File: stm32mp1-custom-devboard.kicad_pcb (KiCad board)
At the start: 4 copper layers, 120 x 72 mm, 50 parts, among them Con1 52746-0671, Con2 505110-2491, Con3 2041119-1, U1 TPS61169DCKR, U2 MCP1703T-3302E, U3 ST1S10PHR, U4 ST1S09IPUR, U5 STM32F103C(8-B)Tx

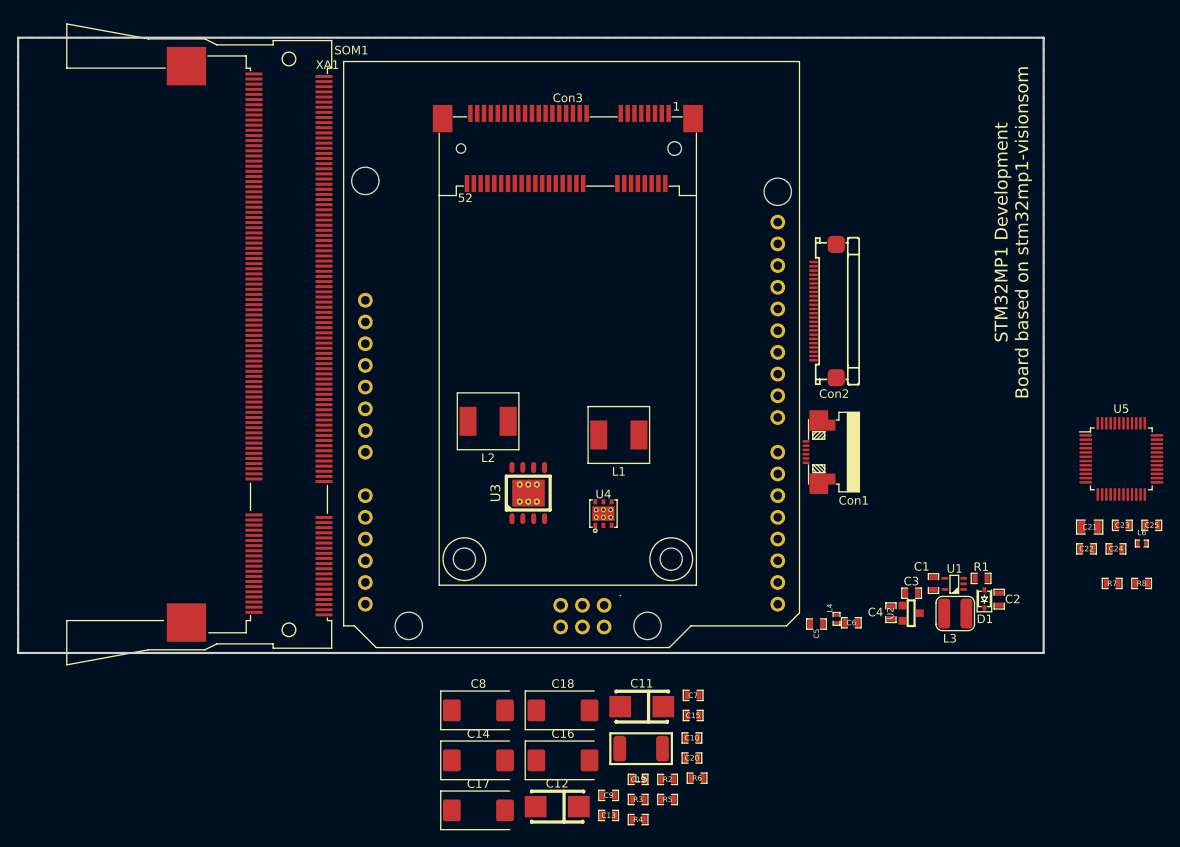
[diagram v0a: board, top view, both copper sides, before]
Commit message: Finished work at st-link, figurated elements on pcb
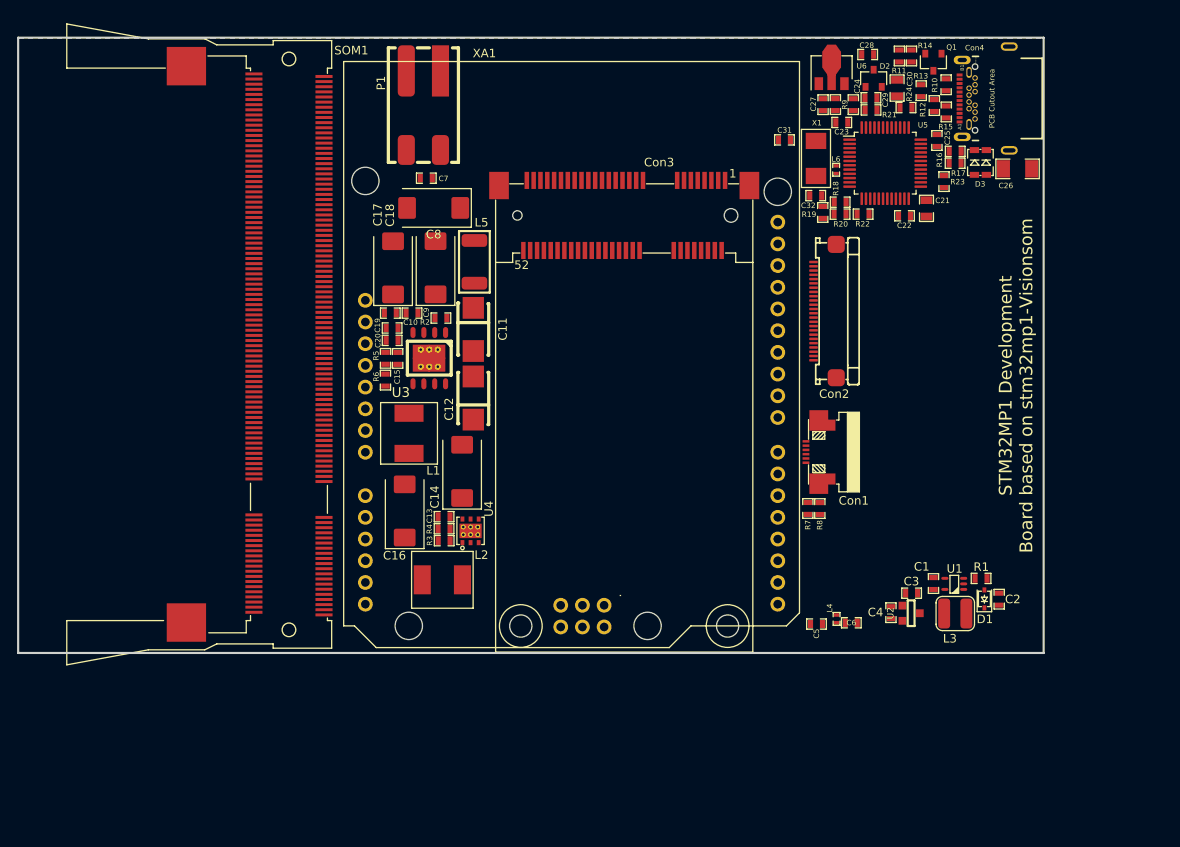
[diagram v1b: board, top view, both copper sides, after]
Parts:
- added C26: 1nF/2kV, Capacitors_Smd_1206:1nF_2kV_1206, F.Cu at (210.1, 81.8)
- added C27: 100n/50V, Capacitors_Smd_0603:100nF_0603, F.Cu at (187.3, 74.2)
- added C28: 100nF/50V, Capacitors_Smd_0603:100nF_0603, F.Cu at (192.5, 68.4)
- added C29: 100nF/50V, Capacitors_Smd_0603:100nF_0603, F.Cu at (192.9, 73.4)
- added C30: 10uF/6V3, Capacitors_Smd_0805:10uF_0805, F.Cu at (196.0, 72.3)
- added C31: 20pF/50V, Capacitors_Smd_0603:20pF_0603, F.Cu at (182.8, 78.4)
- added C32: 20pF/50V, Capacitors_Smd_0603:20pF_0603, F.Cu at (186.4, 84.9)
- added Con4: USB_C_Wurth_632723130112, Connector_USB:USB_C_632723130112, F.Cu at (207.8, 73.5)
- added D2: BAT54C, Diodes:BAT54C, F.Cu at (193.2, 71.2)
- added D3: HSMF-C155, Diodes:HSMF-C155, F.Cu at (205.7, 81.0)
- added P1: Main Power Supply, Smd_Connectors:2060-452_998-404, F.Cu at (140.5, 74.3)
- added Q1: BC847B, Transistor_Bipolar:BC847B_SOT23, F.Cu at (200.2, 69.3)
- added R10: 10k, Resistor_Smd_0603:10k_0603, F.Cu at (201.7, 71.9)
- added R11: 36k, Resistor_Smd_0603:36k_0603, F.Cu at (196.2, 68.5)
- added R12: 22R, Resistor_Smd_0603:22R_0603, F.Cu at (200.3, 74.3)
- added R13: 1k5, Resistor_Smd_0603:1k5_0603, F.Cu at (198.8, 72.6)
- added R14: 100R, Resistor_Smd_0603:100R_0603, F.Cu at (197.6, 68.5)
- added R15: 22R, Resistor_Smd_0603:22R_0603, F.Cu at (201.7, 75.1)
- added R16: 220R, Resistor_Smd_0603:220R_0603, F.Cu at (202.8, 79.7)
- added R17: 220R, Resistor_Smd_0603:220R_0603, F.Cu at (202.8, 81.1)
- added R18: 10k, Resistor_Smd_0603:10k_0603, F.Cu at (189.3, 85.7)
- added R19: 4k7, Resistor_Smd_0603:4k7_0603, F.Cu at (187.3, 86.9)
- added R20: 10k, Resistor_Smd_0603:10k_0603, F.Cu at (189.3, 87.1)
- added R21: 100k, Resistor_Smd_0603:100k_0603, F.Cu at (192.9, 74.9)
- added R22: 4k7, Resistor_Smd_0603:4k7_0603, F.Cu at (192.0, 87.1)
- added R23: 100R, Resistor_Smd_0603:100R_0603, F.Cu at (201.4, 83.2)
- added R24: 0R, Resistor_Smd_0603:0R_0603, F.Cu at (197.0, 74.6)
- added R9: 100k, Resistor_Smd_0603:100k_0603, F.Cu at (188.7, 74.2)
- added U6: MCP1700T-3302E_MB, Linear:MCP1700T-3302E_MB_SOT89, F.Cu at (188.3, 70.3)
- added X1: 8.000MHZ, Resonators:ABM3AIG-8.000MHZ-8-1R-T, F.Cu at (186.5, 80.5)
- moved C7 68.1 mm to (140.9, 82.8), turned to 180 degrees
- moved C17 64.3 mm to (137.0, 93.3), turned to 90 degrees
- moved R5 61.3 mm to (136.1, 103.9), turned to 90 degrees
- moved C10 61.0 mm to (136.7, 98.6), turned to 180 degrees
- moved C9 60.9 mm to (139.2, 98.6), turned to 180 degrees
- moved C24 60.4 mm to (190.8, 74.2), turned to 90 degrees
- moved L5 60.2 mm to (146.5, 92.6), turned to 270 degrees
- moved C20 60.2 mm to (136.9, 101.8)
- moved C19 60.2 mm to (136.9, 100.4)
- moved R2 60.1 mm to (142.6, 99.2), turned to 180 degrees
- moved R6 59.2 mm to (136.1, 106.5), turned to 270 degrees
- moved C8 59.0 mm to (141.7, 86.3), turned to 180 degrees
- moved C23 57.4 mm to (189.5, 76.3), turned to 180 degrees
- moved L6 56.5 mm to (188.8, 81.9), turned to 90 degrees
- moved C15 54.2 mm to (137.5, 103.9), turned to 90 degrees
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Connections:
- C21 pad 1: Net-(C21-Pad1) -> 3V3
- C22 pad 1: Net-(C21-Pad1) -> 3V3
- C23 pad 1: Net-(C21-Pad1) -> 3V3
- C24 pad 1: Net-(C21-Pad1) -> 3V3
- C25 pad 1: Net-(C21-Pad1) -> 3V3
- L6 pad 2: Net-(C21-Pad1) -> 3V3
- U5 pad 1: Net-(C21-Pad1) -> 3V3
- U5 pad 10: (no net) -> Net-(R19-Pad2)
- U5 pad 2: (no net) -> Net-(R20-Pad1)
- U5 pad 20: (no net) -> GND
- U5 pad 24: Net-(C21-Pad1) -> 3V3
- U5 pad 25: (no net) -> Net-(R23-Pad2)
- U5 pad 27: (no net) -> /STLink Module/JTMS
- U5 pad 3: (no net) -> Net-(R18-Pad1)
- U5 pad 30: (no net) -> Net-(R16-Pad2)
- U5 pad 32: (no net) -> Net-(R12-Pad1)
- U5 pad 33: (no net) -> Net-(R15-Pad1)
- U5 pad 36: Net-(C21-Pad1) -> 3V3
- U5 pad 38: (no net) -> Net-(R14-Pad2)
- U5 pad 39: (no net) -> Net-(R24-Pad2)
- U5 pad 44: (no net) -> Net-(R21-Pad2)
- U5 pad 48: Net-(C21-Pad1) -> 3V3
- U5 pad 5: (no net) -> Net-(C31-Pad2)
- U5 pad 6: (no net) -> Net-(C32-Pad2)
- U5 pad 7: (no net) -> Net-(C27-Pad1)
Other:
- board text added: "STM32MP1 Development Board based on stm32mp1-Visionsom"
- board text removed: "STM32MP1 Development Board based on stm32mp1-visionsom"
